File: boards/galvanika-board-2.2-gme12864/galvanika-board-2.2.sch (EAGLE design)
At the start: 184 parts, among them IC1 LM358D, IC2 LM358D, IC3 LM358D

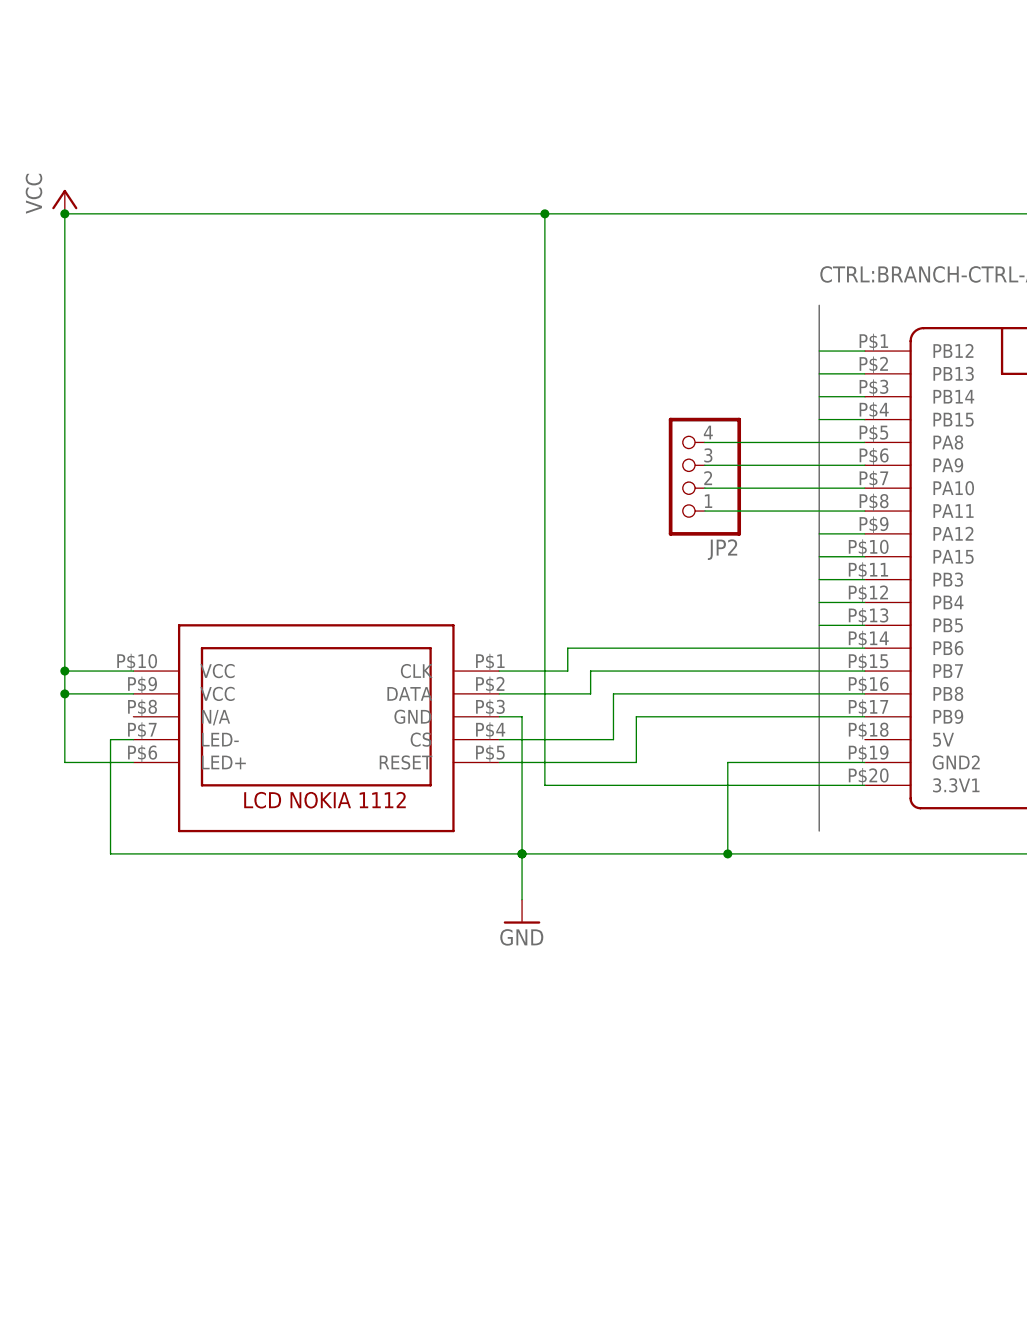
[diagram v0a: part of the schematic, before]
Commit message: Boards V2.2
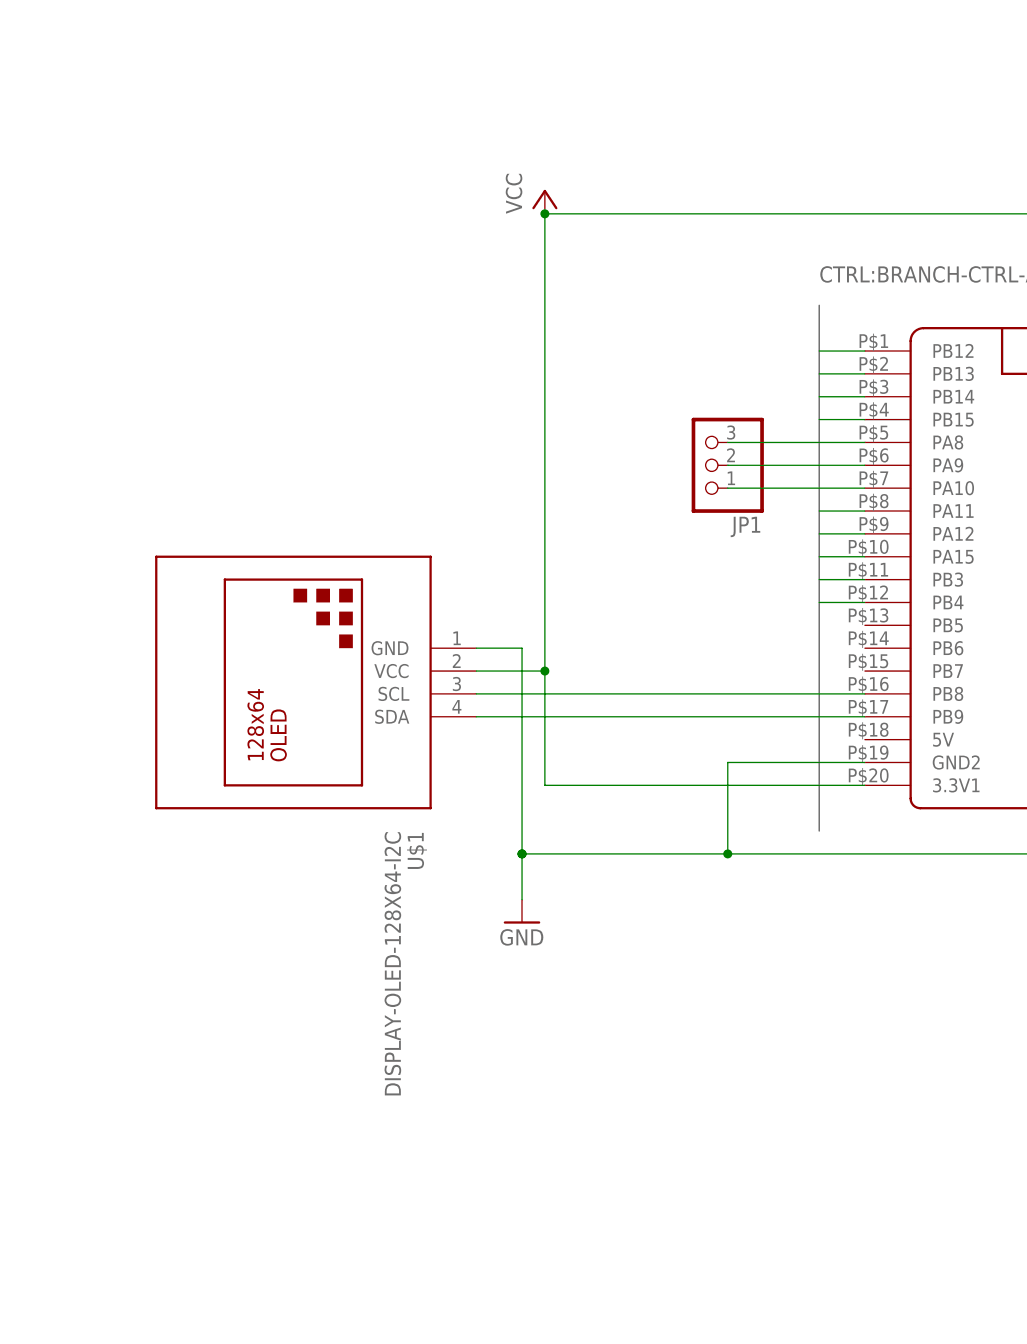
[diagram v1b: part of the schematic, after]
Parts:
- removed HG1: WD-G0906WY-BOARD, dragberry:WD-G0906WY-BOARD
- removed JP2: (no value), pinhead:PINHD-1X4
- added JP1: (no value), pinhead:PINHD-1X3
- added U$1: DISPLAY-OLED-128X64-I2C, diy-modules:DISPLAY-OLED-128X64-I2C
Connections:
- removed net N$45: DD1.PA9, JP2.3
- removed net N$48: DD1.PA10, JP2.2
- removed net N$49: DD1.PA11, JP2.1
- removed net N$95: DD1.PB8, HG1.CS
- removed net N$96: DD1.PB9, HG1.RESET
- new net N$77: DD1.PB8, U$1.SCL
- new net N$80: DD1.PB9, U$1.SDA
- net BRANCH-CTRL-A: now also DD1.PA12; no longer DD1.PA15
- net BRANCH-CTRL-B: now also DD1.PA11; no longer DD1.PA12
- net GND: now also U$1.GND; no longer HG1.GND, HG1.LED-
- net MODE-CTRL-A: now also DD1.PB4; no longer DD1.PB5
- net MODE-CTRL-B: now also DD1.PB3; no longer DD1.PB4
- net MODE-CTRL-C: now also DD1.PA15; no longer DD1.PB3
- net N$11: now also DD1.PA9, JP1.2; no longer DD1.PB6, HG1.CLK
- net N$2: now also DD1.PA8, JP1.3; no longer DD1.PB7, HG1.DATA
- net N$35: now also DD1.PA10, JP1.1; no longer DD1.PA8, JP2.4
- net VCC: now also U$1.VCC; no longer HG1.LED+, HG1.VCC@1, HG1.VCC@2
